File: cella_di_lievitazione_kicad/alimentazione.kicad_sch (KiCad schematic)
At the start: 8 parts, among them J1 Screw_Terminal_01x02, J2 USB_C_Receptacle_PowerOnly_24P, SW2 SW_Nidec_CAS-120A1, U1 CYPD3177-24LQ

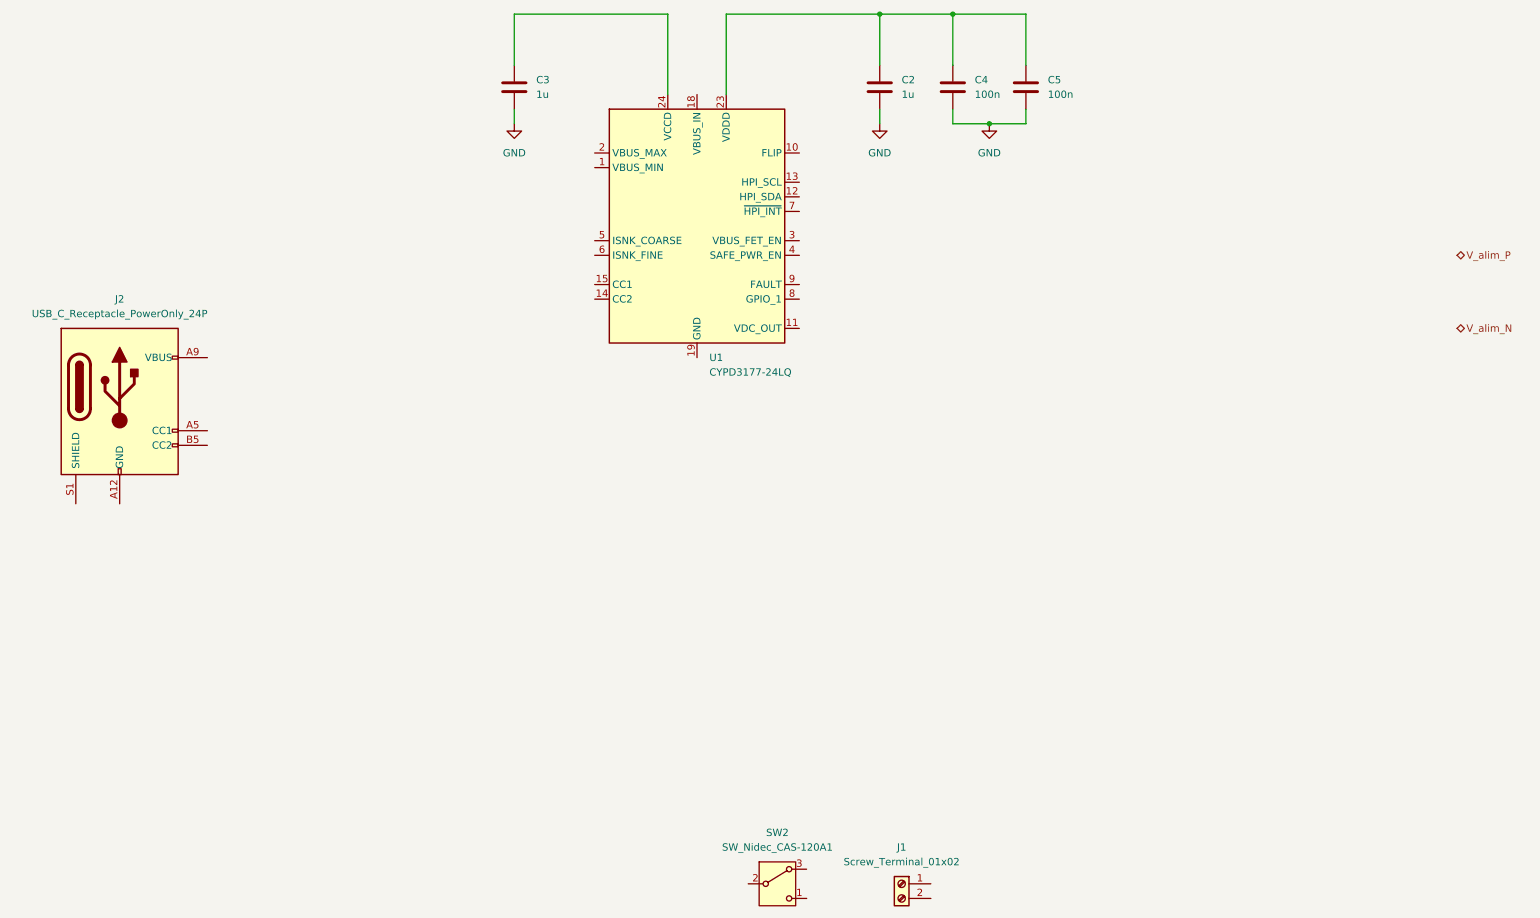
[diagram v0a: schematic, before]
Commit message: no message
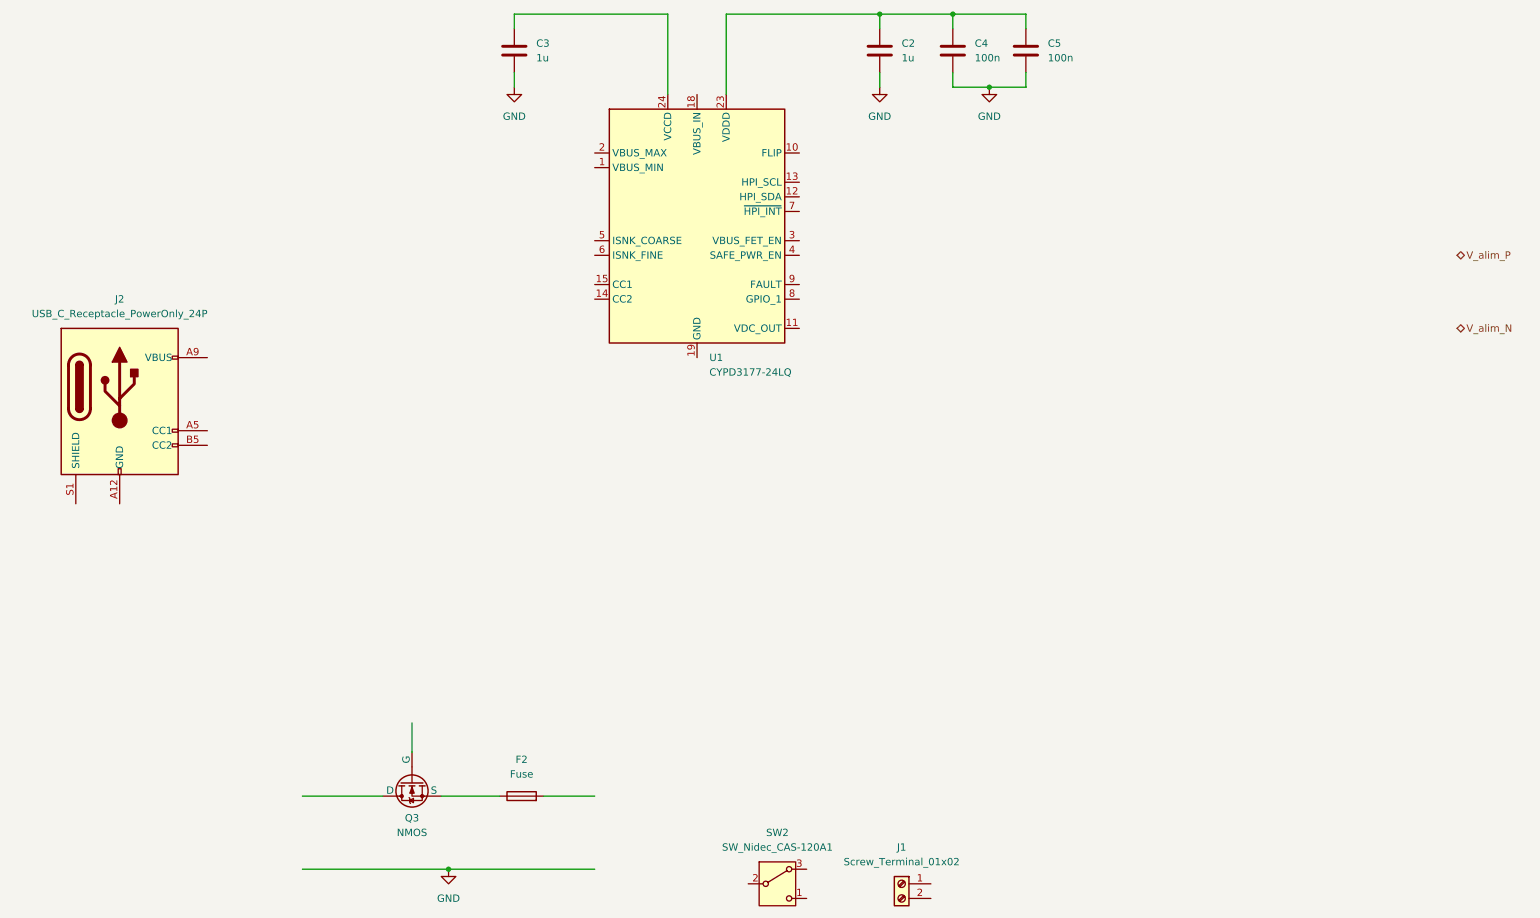
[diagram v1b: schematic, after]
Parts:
- added F2: Fuse, symbol Device:Fuse
- added Q3: NMOS, symbol Simulation_SPICE:NMOS
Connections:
- new net: F2.1, Q3.3 (S)
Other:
- moved on the sheet: C2, C3, C4, C5
